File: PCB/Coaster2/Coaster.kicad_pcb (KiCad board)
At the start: 2 copper layers, 100 x 100 mm, 279 parts, among them J1 Reset, J2 TC2030-USB-NL-DS, J3 USB-C-Socket-H, U1 ICS43434_MEMS_Mic, U2 ESP32-S3-MINI-1, U3 MD8942

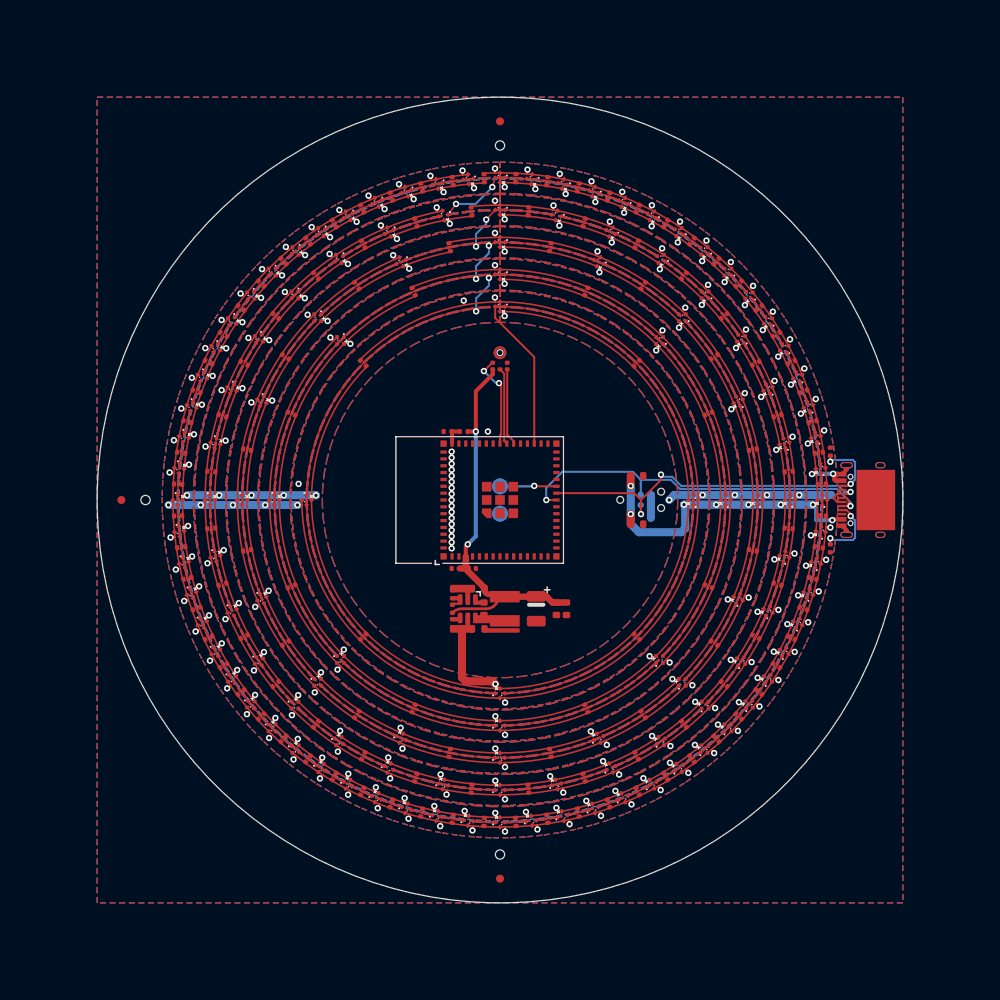
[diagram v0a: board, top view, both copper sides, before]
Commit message: Final, and spacers
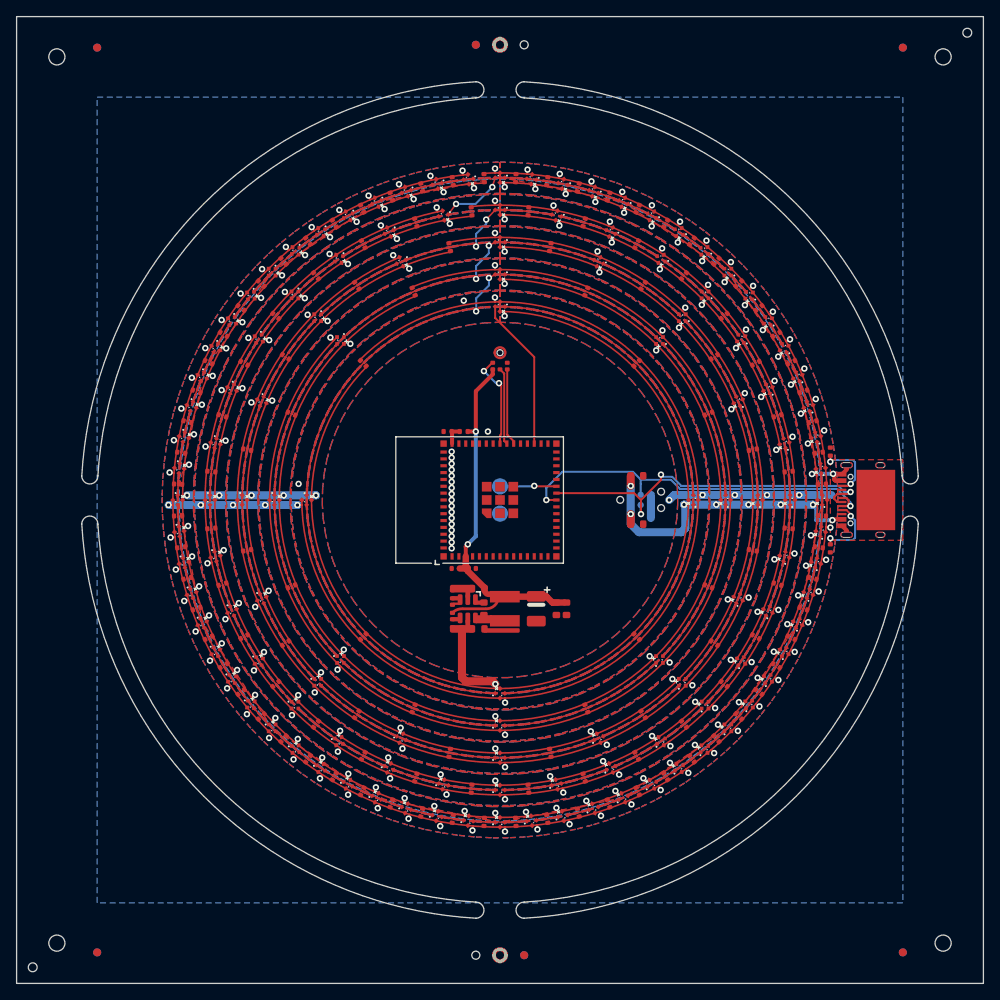
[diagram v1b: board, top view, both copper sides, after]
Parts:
- removed FID1, FID2, FID3: Fiducial, RevK:Hole-Tooling
- removed FID4, FID5, FID6: Fiducial, Fiducial:Fiducial_1mm_Mask2mm
- added PCB1: 120x120, RevK:PCB120120, F.Cu at (100.0, 100.0)
- added V1: ~, RevK:VCUT120N, F.Cu at (100.0, 50.1)
- added V2: ~, RevK:VCUT120N, F.Cu at (100.0, 149.9)
- added V3: ~, RevK:VCUT120N, F.Cu at (149.9, 100.0)
- added V4: ~, RevK:VCUT120N, F.Cu at (50.1, 100.0)
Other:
- board size 100 x 100 mm -> 120 x 120 mm
- board text added: "37"
- board text added: "40 41 42"
- board text added: "LED"
- board text added: "WS SD SCK"
- board text removed: "37 40 41 42"
- board text removed: "LED WS SD SCK"
